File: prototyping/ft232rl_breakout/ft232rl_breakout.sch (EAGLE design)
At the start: 17 parts, among them J1 USB, U1 FT232RL

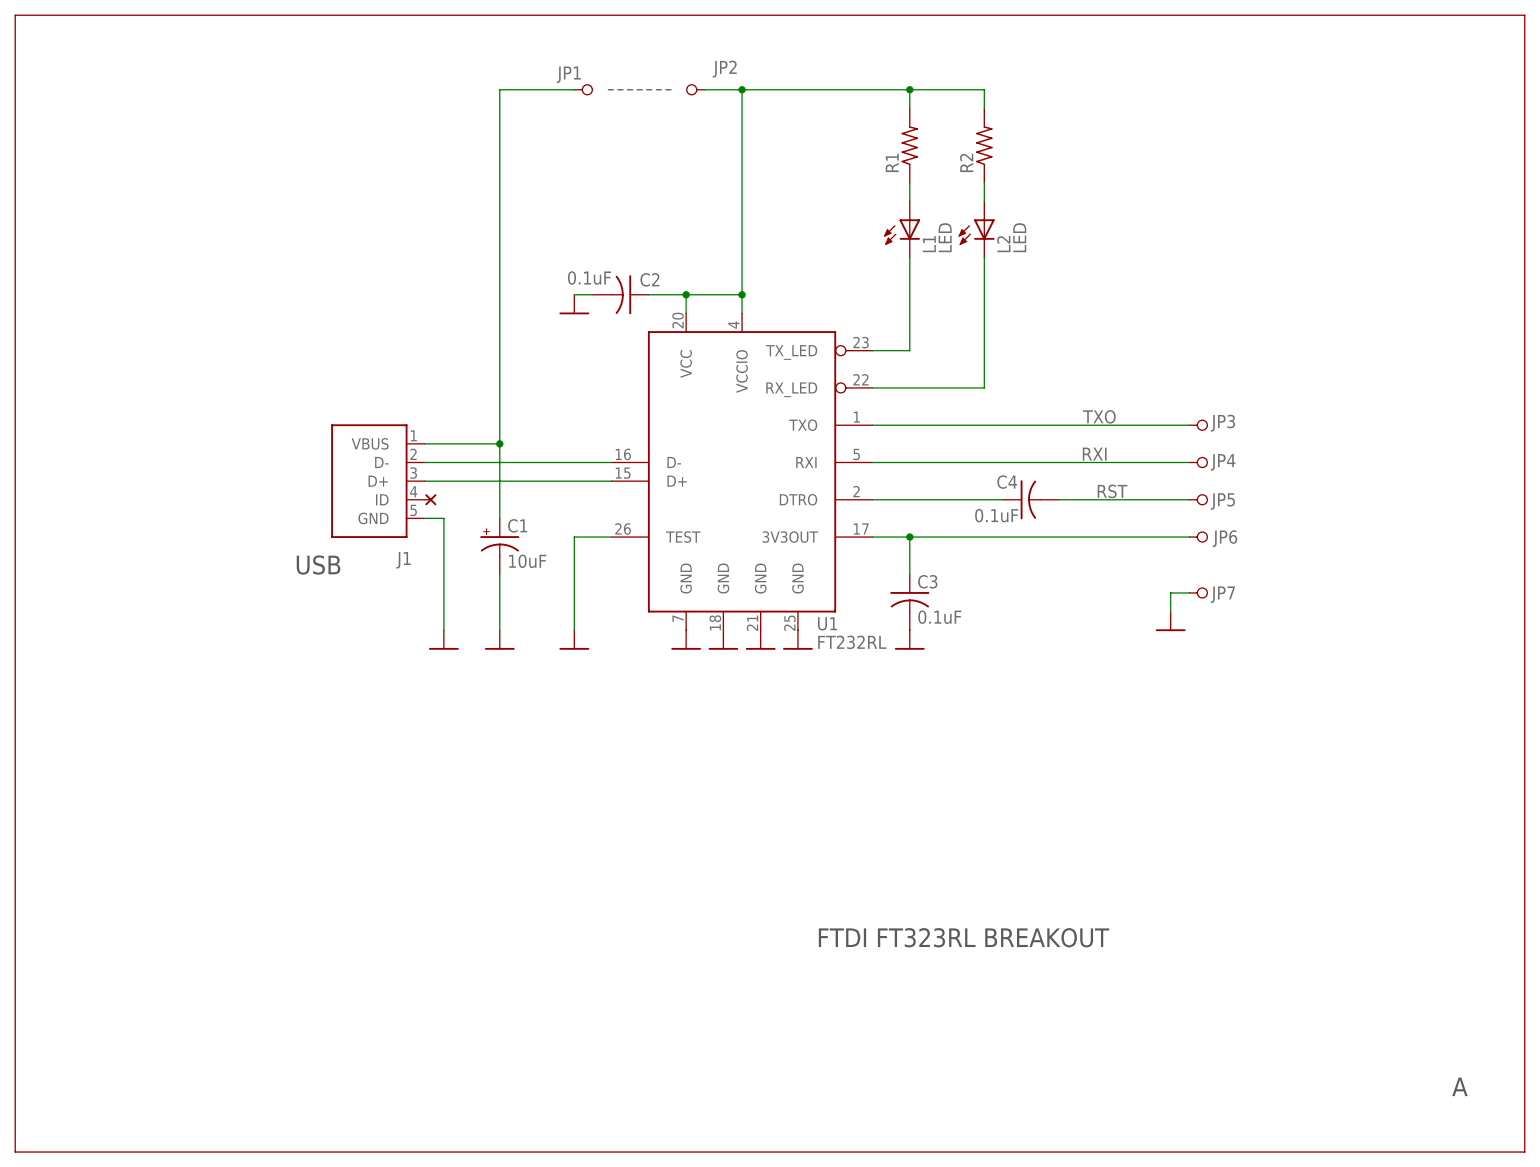
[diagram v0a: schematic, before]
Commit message: Performed final auto routing.
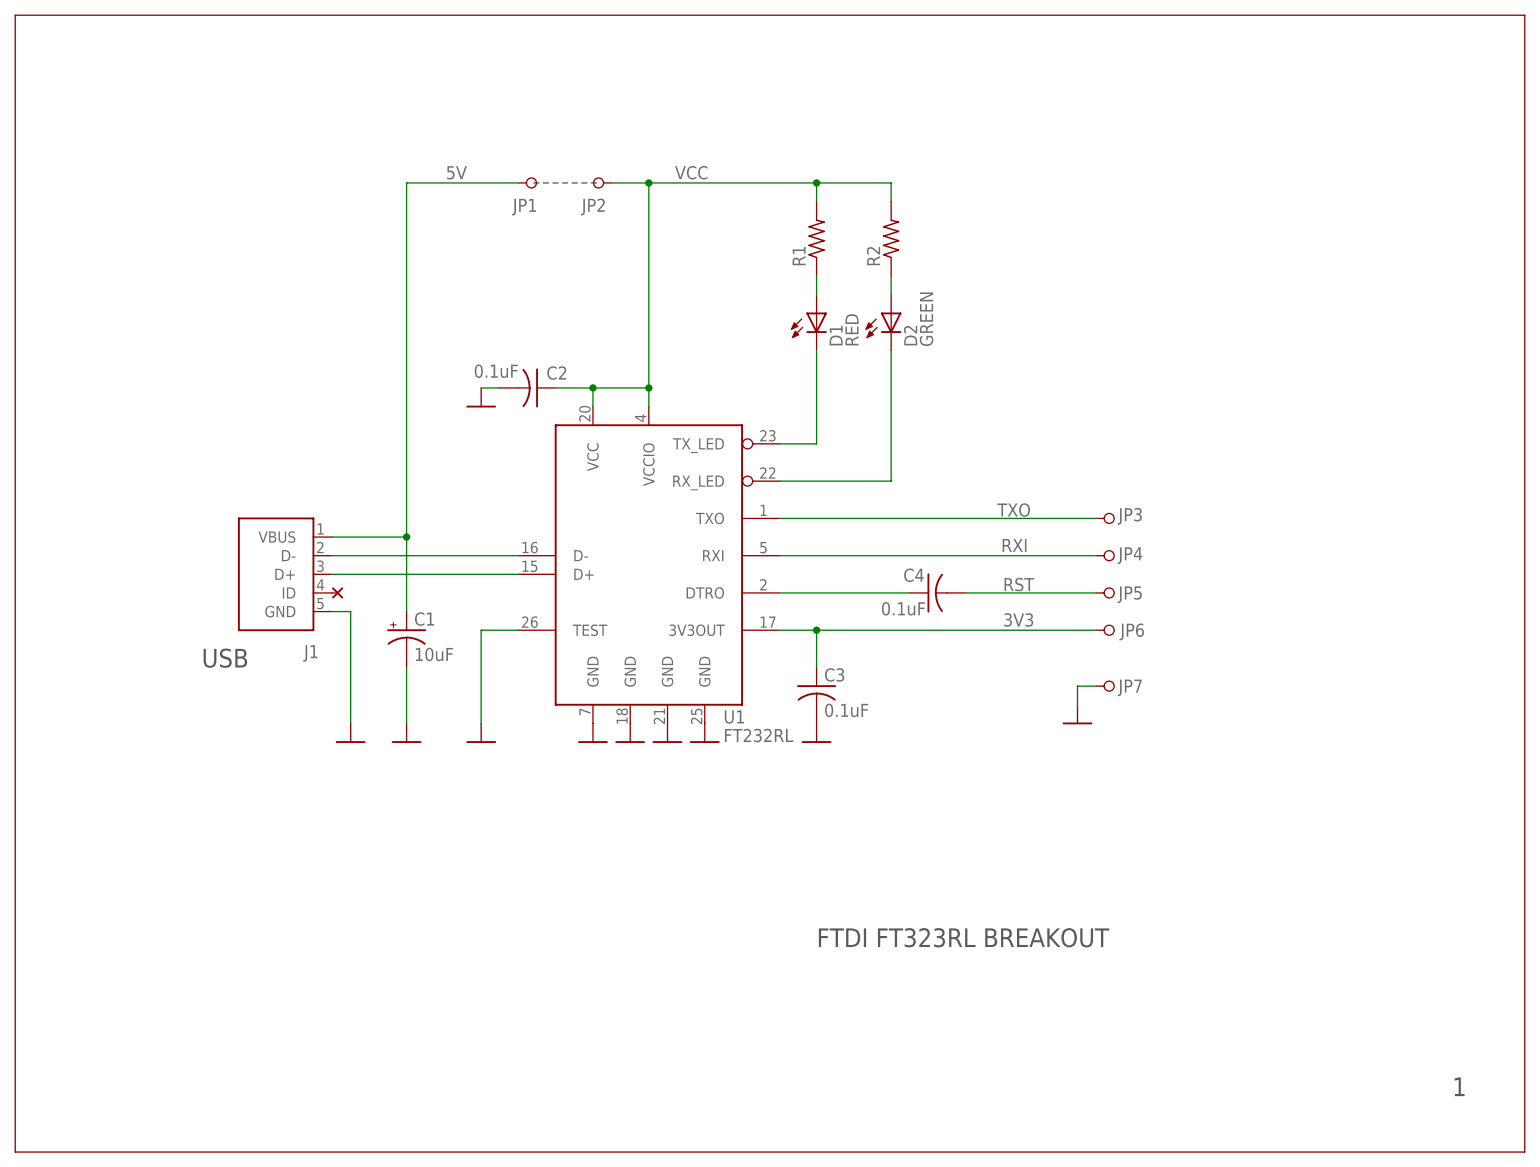
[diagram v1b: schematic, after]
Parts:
- removed L1, L2: LED, ft232rl_breakout:LED
- added D1: RED, ft232rl_breakout:LED
- added D2: GREEN, ft232rl_breakout:LED
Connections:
- net N$1 renamed VCC
- net N$16 renamed 3V3
- net VUSB renamed 5V
- net N$2: now also D1.C; no longer L1.C
- net N$3: now also D2.C; no longer L2.C
- net N$4: now also D1.A; no longer L1.A
- net N$5: now also D2.A; no longer L2.A
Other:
- note added: "1"
- note removed: "A"
- moved on the sheet: C1, C2, C3, C4, J1, JP1, JP2, JP3, JP4, JP5, JP6, JP7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
